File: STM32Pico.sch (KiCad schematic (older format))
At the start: 25 parts, among them J1 2.54mm header 01x20, J2 2.54mm header 01x20, SW1 Boot Mode, SW2 Reset Switch, U1 STM32F411CEUx, U2 XC6206PxxxMR, X1 ECS-2520MV-xxx-xx

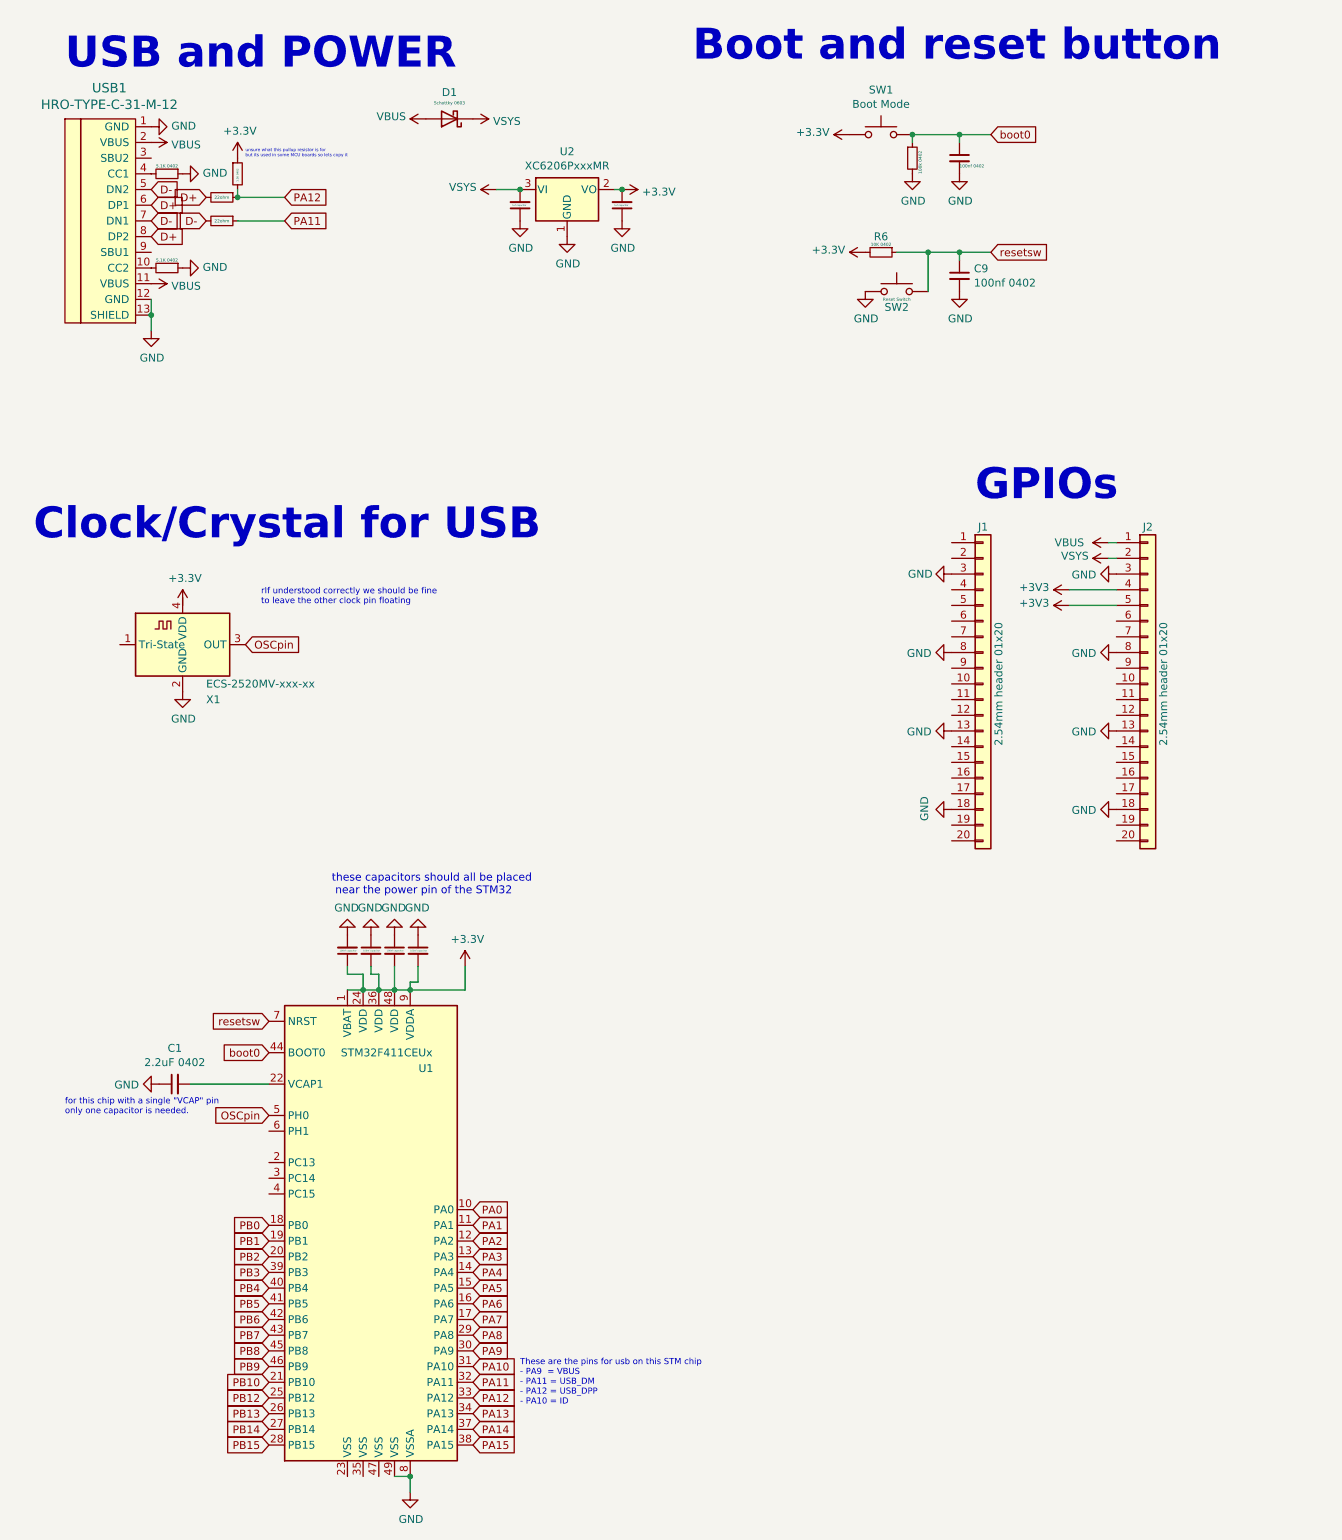
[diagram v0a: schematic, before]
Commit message: finished up board design, likely needs some check overs and revision.
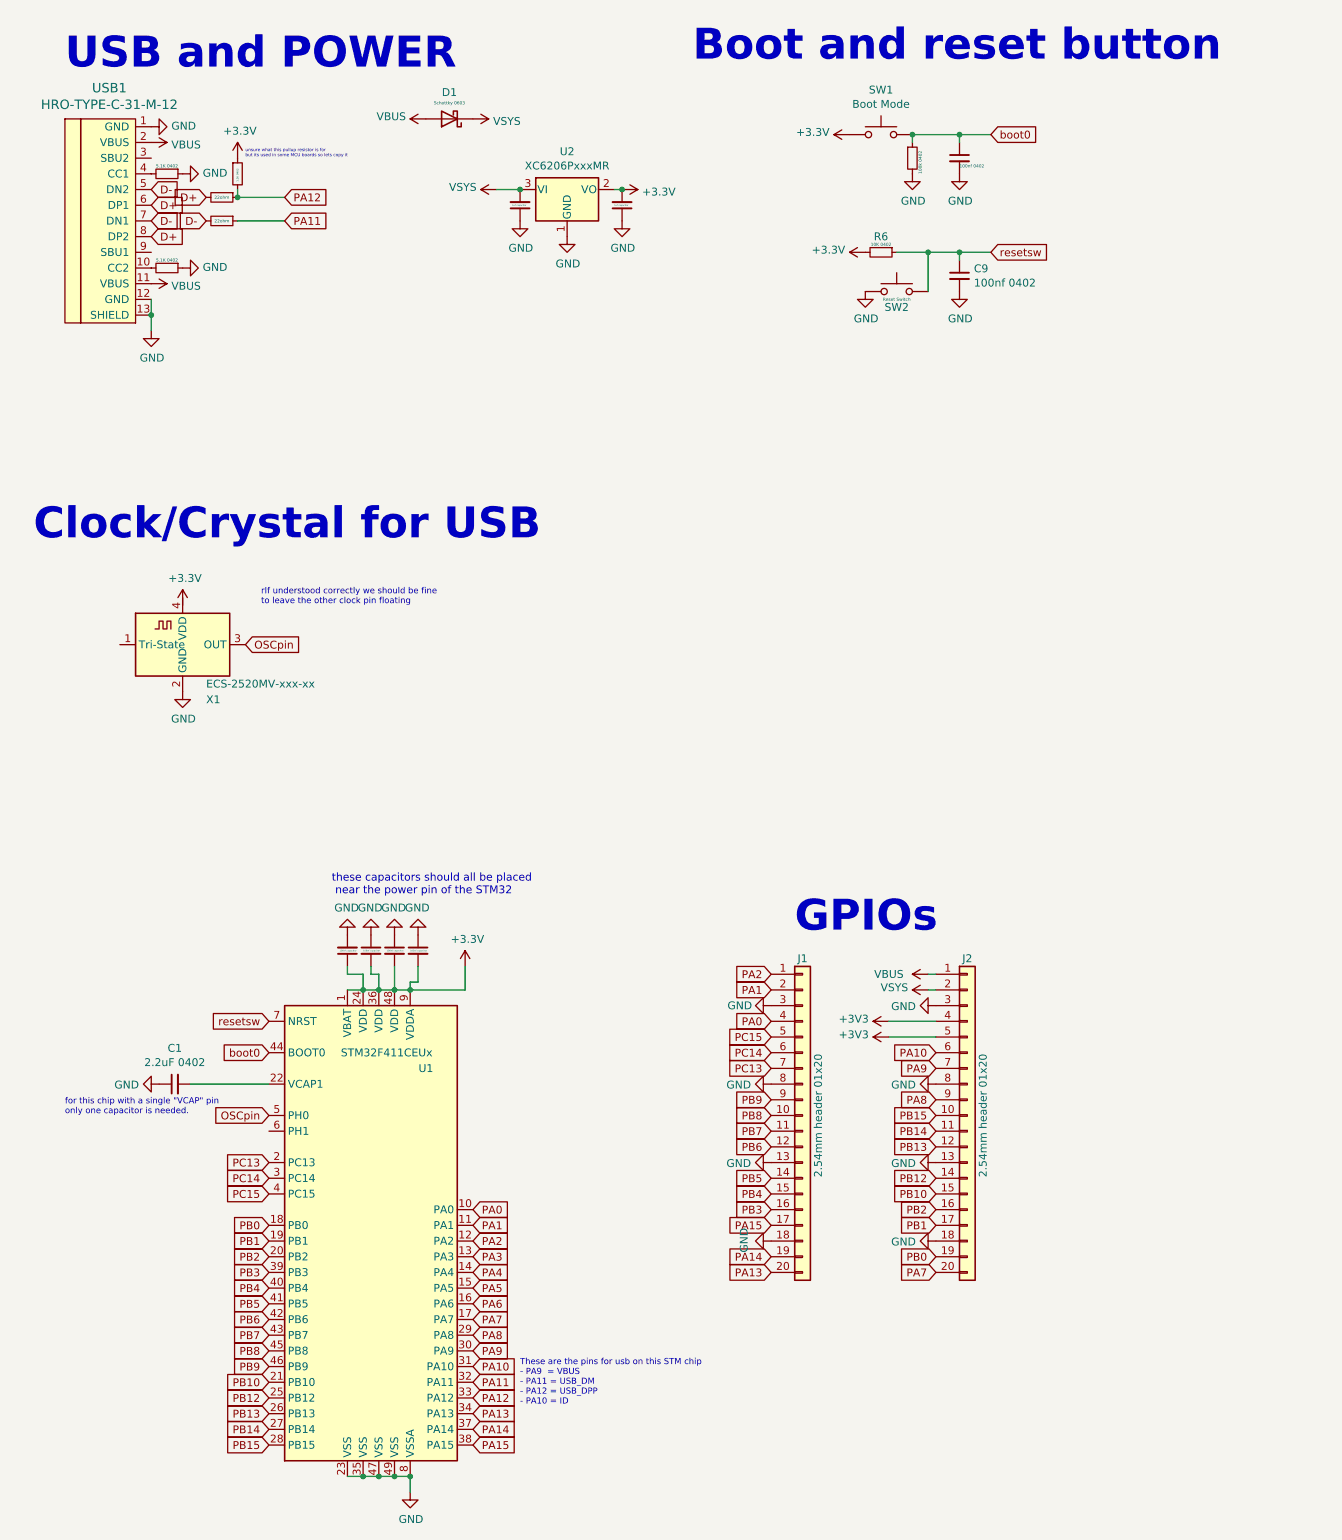
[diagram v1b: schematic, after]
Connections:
- net GND: now also U1.23 (VSS), U1.35 (VSS), U1.47 (VSS)
- net PA0: now also J1.4 (Pin_4)
- net PA1: now also J1.2 (Pin_2)
- net PA10: now also J2.6 (Pin_6)
- net PA13: now also J1.20 (Pin_20)
- net PA14: now also J1.19 (Pin_19)
- net PA15: now also J1.17 (Pin_17)
- net PA2: now also J1.1 (Pin_1)
- net PA7: now also J2.20 (Pin_20)
- net PA8: now also J2.9 (Pin_9)
- net PA9: now also J2.7 (Pin_7)
- net PB0: now also J2.19 (Pin_19)
- net PB1: now also J2.17 (Pin_17)
- net PB10: now also J2.15 (Pin_15)
- net PB12: now also J2.14 (Pin_14)
- net PB13: now also J2.12 (Pin_12)
- net PB14: now also J2.11 (Pin_11)
- net PB15: now also J2.10 (Pin_10)
- net PB2: now also J2.16 (Pin_16)
- net PB3: now also J1.16 (Pin_16)
- net PB4: now also J1.15 (Pin_15)
- net PB5: now also J1.14 (Pin_14)
- net PB6: now also J1.12 (Pin_12)
- net PB7: now also J1.11 (Pin_11)
- net PB8: now also J1.10 (Pin_10)
- net PB9: now also J1.9 (Pin_9)
- net PC15: now reaches J1.5 (Pin_5)
- net PC15: now also U1.4 (PC15)
- net PC14: now reaches J1.6 (Pin_6)
- net PC14: now also U1.3 (PC14)
- net PC13: now reaches J1.7 (Pin_7)
- net PC13: now also U1.2 (PC13)
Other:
- moved on the sheet: J1, J2
